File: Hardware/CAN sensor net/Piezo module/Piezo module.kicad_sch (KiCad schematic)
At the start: 28 parts, among them SW1 SW_Push, SW2 SW_SPDT, U1 STM32F103C8Tx, U2 SN65HVD230, U3 W25Q32FVSSIG, Y1 16MHz

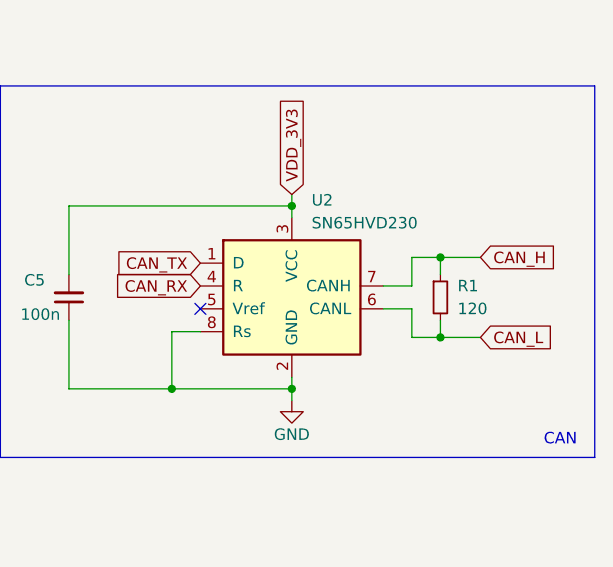
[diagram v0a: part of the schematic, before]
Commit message: added solder jumpers for 120R CAN
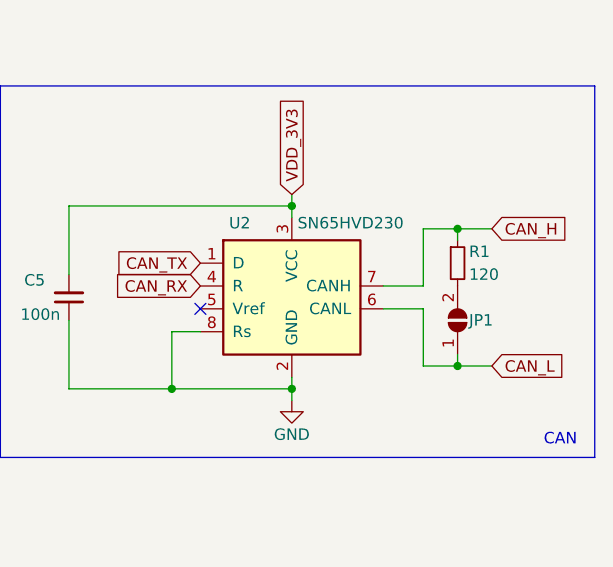
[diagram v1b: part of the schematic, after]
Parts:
- added JP1: SolderJumper_2_Open, symbol Jumper:SolderJumper_2_Open
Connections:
- net CAN_L: now also JP1.1 (A); no longer R1.2
- new net: JP1.2 (B), R1.2
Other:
- moved on the sheet: R1
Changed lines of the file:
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@@
 	)
 	(junction
-		(at 163.83 66.675)
+		(at 265.43 144.78)
 		(diameter 0)
 		(color 0 0 0 0)
 	)
 	(junction
-		(at 229.235 43.18)
+		(at 163.83 66.675)
 		(diameter 0)
 		(color 0 0 0 0)
 	)
 	(junction
-		(at 263.525 132.715)
+		(at 229.235 43.18)
 		(diameter 0)
 		(color 0 0 0 0)
@@
 	)
 	(junction
-		(at 263.525 141.605)
-		(diameter 0)
-		(color 0 0 0 0)
-	)
-	(junction
 		(at 66.04 159.385)
 		(diameter 0)
@@
 	)
 	(junction
+		(at 265.43 129.54)
+		(diameter 0)
+		(color 0 0 0 0)
+	)
+	(junction
 		(at 233.68 147.32)
 		(diameter 0)
@@
 	(wire
 		(pts
-			(xy 263.525 141.605) (xy 267.97 141.605)
-		)
-		(stroke
-			(width 0)
-			(type default)
-		)
-	)
-	(wire
-		(pts
 			(xy 68.58 159.385) (xy 68.58 155.575)
 		)
@@
 	(wire
 		(pts
-			(xy 260.35 132.715) (xy 263.525 132.715)
+			(xy 261.62 129.54) (xy 265.43 129.54)
 		)
 		(stroke
@@
 	(wire
 		(pts
-			(xy 263.525 139.7) (xy 263.525 141.605)
-		)
-		(stroke
-			(width 0)
-			(type default)
-		)
-	)
-	(wire
-		(pts
 			(xy 146.05 60.325) (xy 146.05 80.645)
 		)
@@
 		)
 	)
-	(polyline
+	(wire
 		(pts
-			(xy 280.035 15.875) (xy 280.035 55.88)
+			(xy 265.43 129.54) (xy 269.24 129.54)
 		)
 		(stroke
@@
 	(polyline
 		(pts
-			(xy 166.37 15.875) (xy 125.73 15.875)
+			(xy 280.035 15.875) (xy 280.035 55.88)
 		)
 		(stroke
@@
 	(polyline
 		(pts
-			(xy 280.035 58.42) (xy 280.035 90.805)
+			(xy 166.37 15.875) (xy 125.73 15.875)
 		)
 		(stroke
@@
 		)
 	)
-	(wire
+	(polyline
 		(pts
-			(xy 72.39 73.025) (xy 72.39 69.215)
+			(xy 280.035 58.42) (xy 280.035 90.805)
 		)
 		(stroke
@@
 	(wire
 		(pts
-			(xy 244.475 36.83) (xy 244.475 35.56)
+			(xy 72.39 73.025) (xy 72.39 69.215)
 		)
 		(stroke
@@
 	(wire
 		(pts
-			(xy 260.35 132.715) (xy 260.35 135.89)
+			(xy 244.475 36.83) (xy 244.475 35.56)
 		)
 		(stroke
@@
 	(wire
 		(pts
-			(xy 263.525 132.715) (xy 267.97 132.715)
+			(xy 261.62 129.54) (xy 261.62 135.89)
 		)
 		(stroke
@@
 	(wire
 		(pts
-			(xy 257.175 138.43) (xy 260.35 138.43)
+			(xy 257.175 138.43) (xy 261.62 138.43)
 		)
 		(stroke
@@
 	(wire
 		(pts
+			(xy 265.43 143.51) (xy 265.43 144.78)
+		)
+		(stroke
+			(width 0)
+			(type default)
+		)
+	)
+	(wire
+		(pts
 			(xy 204.47 74.93) (xy 207.01 74.93)
 		)
@@
 	(wire
 		(pts
+			(xy 265.43 144.78) (xy 269.24 144.78)
+		)
+		(stroke
+			(width 0)
+			(type default)
+		)
+	)
+	(wire
+		(pts
 			(xy 192.405 22.86) (xy 192.405 26.67)
 		)
@@
 	(wire
 		(pts
-			(xy 260.35 141.605) (xy 263.525 141.605)
+			(xy 261.62 144.78) (xy 265.43 144.78)
 		)
 		(stroke
@@
 	(wire
 		(pts
-			(xy 260.35 138.43) (xy 260.35 141.605)
+			(xy 261.62 138.43) (xy 261.62 144.78)
 		)
 		(stroke
@@
 		)
 	)
+	(wire
+		(pts
+			(xy 265.43 129.54) (xy 265.43 130.81)
+		)
+		(stroke
+			(width 0)
+			(type default)
+		)
+	)
 	(polyline
 		(pts
@@
 	(wire
 		(pts
-			(xy 257.175 135.89) (xy 260.35 135.89)
+			(xy 257.175 135.89) (xy 261.62 135.89)
 		)
 		(stroke
@@
 	(wire
 		(pts
-			(xy 263.525 132.715) (xy 263.525 134.62)
-		)
-		(stroke
-			(width 0)
-			(type default)
-		)
-	)
-	(wire
-		(pts
 			(xy 72.39 73.025) (xy 69.85 73.025)
 		)
@@
 	(global_label "CAN_H"
 		(shape input)
-		(at 267.97 132.715 0)
+		(at 269.24 129.54 0)
 		(fields_autoplaced yes)
 		(effects
@@
 		)
 		(property "Intersheetrefs" "${INTERSHEET_REFS}"
-			(at 276.9424 132.715 0)
+			(at 278.2124 129.54 0)
 			(effects
 				(font
@@
 	(global_label "CAN_L"
 		(shape input)
-		(at 267.97 141.605 0)
+		(at 269.24 144.78 0)
 		(fields_autoplaced yes)
 		(effects
@@
 		)
 		(property "Intersheetrefs" "${INTERSHEET_REFS}"
-			(at 276.64 141.605 0)
+			(at 277.91 144.78 0)
 			(effects
 				(font
@@
 	(symbol
 		(lib_id "Device:R_Small")
-		(at 263.525 137.16 0)
+		(at 265.43 133.35 0)
 		(unit 1)
 		(exclude_from_sim no)
@@
 		(on_board yes)
 		(dnp no)
-		(fields_autoplaced yes)
 		(property "Reference" "R1"
-			(at 265.43 135.8899 0)
+			(at 266.7 132.08 0)
 			(effects
 				(font
@@
 		)
 		(property "Value" "120"
-			(at 265.43 138.4299 0)
+			(at 266.7 134.62 0)
 			(effects
 				(font
@@
 		)
 		(property "Footprint" "Resistor_SMD:R_0603_1608Metric"
-			(at 263.525 137.16 0)
+			(at 265.43 133.35 0)
 			(effects
 				(font
@@
 		)
 		(property "Datasheet" "~"
-			(at 263.525 137.16 0)
+			(at 265.43 133.35 0)
 			(effects
 				(font
@@
 		)
 		(property "Description" "Resistor, small symbol"
-			(at 263.525 137.16 0)
+			(at 265.43 133.35 0)
 			(effects
 				(font
@@
 		(on_board yes)
 		(dnp no)
-		(fields_autoplaced yes)
 		(property "Reference" "U2"
-			(at 249.2091 126.365 0)
+			(at 240.03 128.905 0)
 			(effects
 				(font
@@
 		)
 		(property "Value" "SN65HVD230"
-			(at 249.2091 128.905 0)
+			(at 247.65 128.905 0)
 			(effects
 				(font
@@
 					(unit 1)
 				)
+			)
+		)
+	)
+	(symbol
+		(lib_id "Jumper:SolderJumper_2_Open")
+		(at 265.43 139.7 90)
+		(unit 1)
+		(exclude_from_sim no)
+		(in_bom yes)
+		(on_board yes)
+		(dnp no)
+		(property "Reference" "JP1"
+			(at 266.7 139.7 90)
+			(effects
+				(font
+					(size 1.27 1.27)
+				)
+				(justify right)
+			)
+		)
+		(property "Value" "SolderJumper_2_Open"
+			(at 267.97 140.9699 90)
+			(effects
+				(font
+					(size 1.27 1.27)
+				)
+				(justify right)
+				(hide yes)
+			)
+		)
+		(property "Footprint" ""
+			(at 265.43 139.7 0)
+			(effects
+				(font
+					(size 1.27 1.27)
+				)
+				(hide yes)
+			)
+		)
+		(property "Datasheet" "~"
+			(at 265.43 139.7 0)
+			(effects
+				(font
+					(size 1.27 1.27)
+				)
+				(hide yes)
+			)
+		)
+		(property "Description" "Solder Jumper, 2-pole, open"
+			(at 265.43 139.7 0)
+			(effects
+				(font
+					(size 1.27 1.27)
+				)
+				(hide yes)
+			)
+		)
+		(pin "1"
+		)
+		(pin "2"
+		)
+		(instances
+			(project "Piezo module"
+				(path "/0a58466e-2312-402a-82c7-7de62fe91dff"
+					(reference "JP1")
+					(unit 1)
+				)

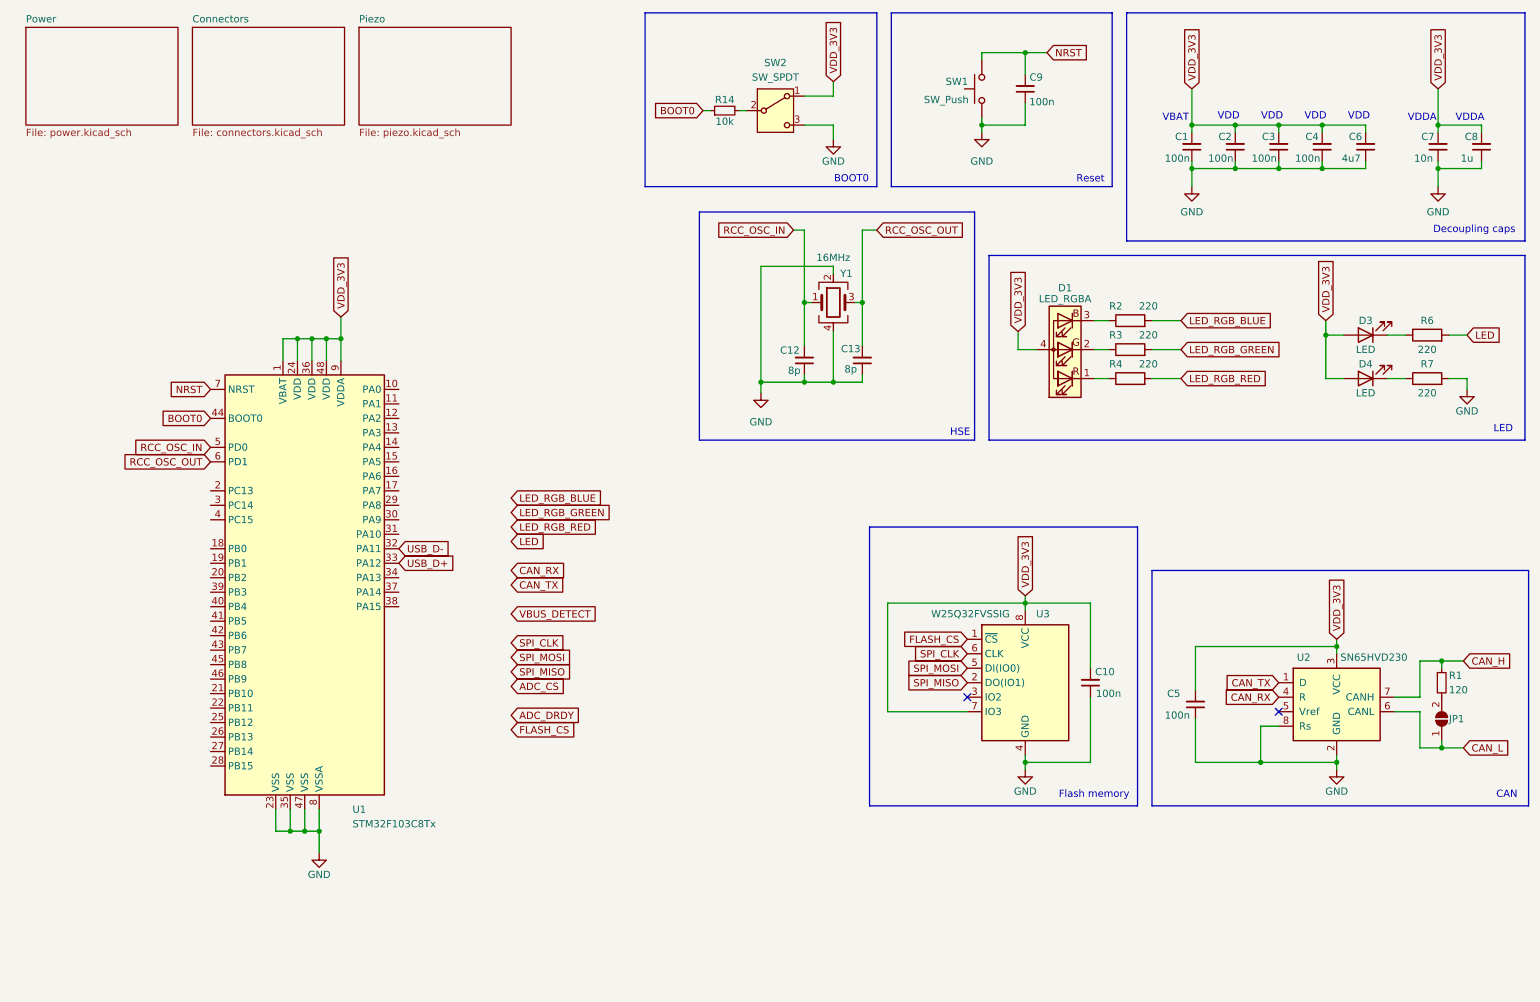
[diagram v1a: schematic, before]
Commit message: updated piezo module
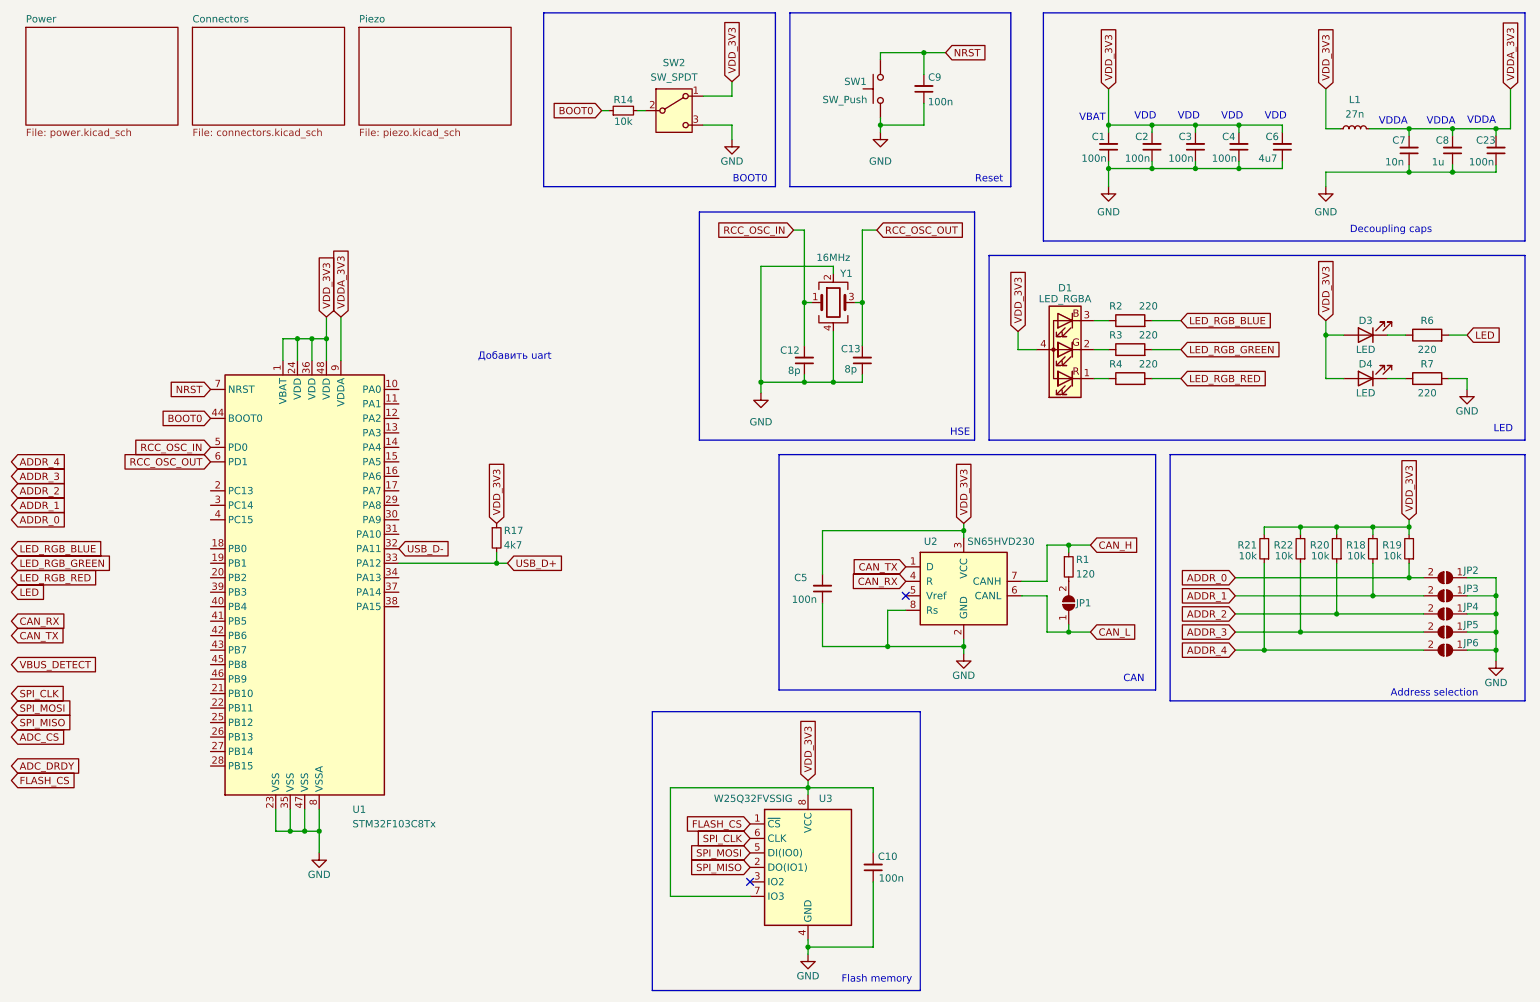
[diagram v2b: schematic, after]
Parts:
- added C23: 100n, Capacitor_SMD:C_0603_1608Metric, symbol Device:C_Small
- added JP2, JP3, JP4, JP5, JP6: SolderJumper_2_Open, Jumper:SolderJumper-2_P1.3mm_Open_RoundedPad1.0x1.5mm, symbol Jumper:SolderJumper_2_Open
- added L1: 27n, symbol Device:L_Small
- added R17: 4k7, symbol Device:R_Small
- added R18, R19, R20, R21, R22: 10k, symbol Device:R_Small
- JP1: footprint (none) -> Jumper:SolderJumper-2_P1.3mm_Open_RoundedPad1.0x1.5mm
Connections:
- net GND: now also C23.1, JP2.1 (A), JP3.1 (A), JP4.1 (A), JP5.1 (A), JP6.1 (A)
- net USB_D+: now also R17.2
- net VDD_3V3: now also L1.1, R17.1, R18.2, R19.2, R20.2, R21.2, R22.2; no longer C7.2, C8.2, U1.9 (VDDA)
- new net ADDR_0: JP2.2 (B), R19.1
- new net ADDR_1: JP3.2 (B), R18.1
- new net ADDR_2: JP4.2 (B), R20.1
- new net ADDR_3: JP5.2 (B), R22.1
- new net ADDR_4: JP6.2 (B), R21.1
- new net VDDA_3V3: C23.2, C7.2, C8.2, L1.2, U1.9 (VDDA)
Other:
- note added: "Address selection"
- note added: "Добавить uart"
- moved on the sheet: C1, C10, C2, C3, C4, C5, C6, C7, C8, C9, JP1, R1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

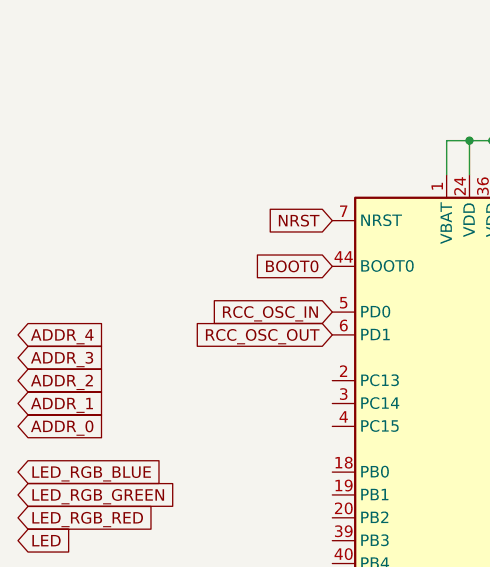
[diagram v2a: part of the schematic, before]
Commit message: added band pass filter to piezo board
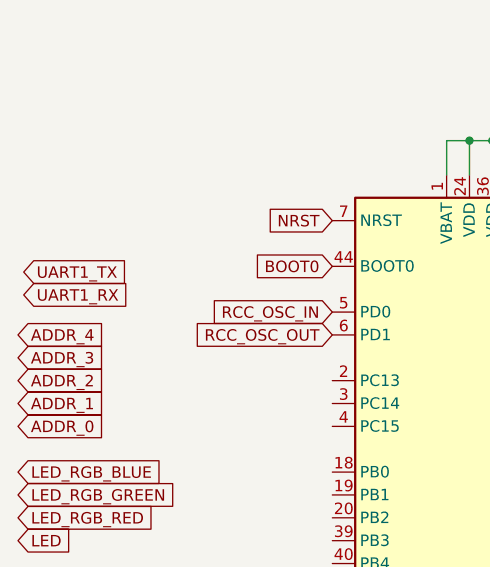
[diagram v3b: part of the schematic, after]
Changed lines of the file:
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@@
+		)
+	)
+	(global_label "UART1_RX"
+		(shape input)
+		(at 15.24 90.17 0)
+		(fields_autoplaced yes)
+		(effects
+			(font
+				(size 1.27 1.27)
+			)
+			(justify left)
+		)
+		(property "Intersheetrefs" "${INTERSHEET_REFS}"
+			(at 27.5385 90.17 0)
+			(effects
+				(font
+					(size 1.27 1.27)
+				)
+				(justify left)
+				(hide yes)
+			)
 		)
 	)
@@
 			(effects
 				(font
+					(size 1.27 1.27)
+				)
+				(justify left)
+				(hide yes)
+			)
+		)
+	)
+	(global_label "UART1_TX"
+		(shape input)
+		(at 15.24 87.63 0)
+		(fields_autoplaced yes)
+		(effects
+			(font
+				(size 1.27 1.27)
+			)
+			(justify left)
+		)
+		(property "Intersheetrefs" "${INTERSHEET_REFS}"
+			(at 27.2361 87.63 0)
+			(effects
+				(font
